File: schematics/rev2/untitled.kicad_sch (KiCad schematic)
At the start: 94 parts, among them SW1 KS-33, SW10 KS-33, SW11 KS-33, SW12 KS-33, SW13 KS-33, SW14 KS-33, SW15 KS-33, SW16 KS-33, SW17 KS-33, SW18 KS-33, SW19 KS-33, SW2 KS-33, SW20 KS-33, SW21 KS-33, SW22 KS-33, SW23 KS-33, SW24 KS-33, SW25 KS-33, SW26 KS-33, SW27 KS-33, SW28 KS-33, SW29 KS-33, SW3 KS-33, SW30 KS-33, SW31 KS-33, SW32 KS-33, SW33 KS-33, SW34 KS-33, SW35 KS-33, SW36 KS-33, SW37 KS-33, SW38 KS-33, SW39 KS-33, SW4 KS-33, SW40 KS-33, SW41 KS-33, SW42 KS-33, SW43 KS-33, SW44 KS-33, SW45 KS-33, SW46 KS-33, SW48 KS-33, SW5 KS-33, SW6 KS-33, SW7 KS-33, SW8 KS-33, SW9 KS-33

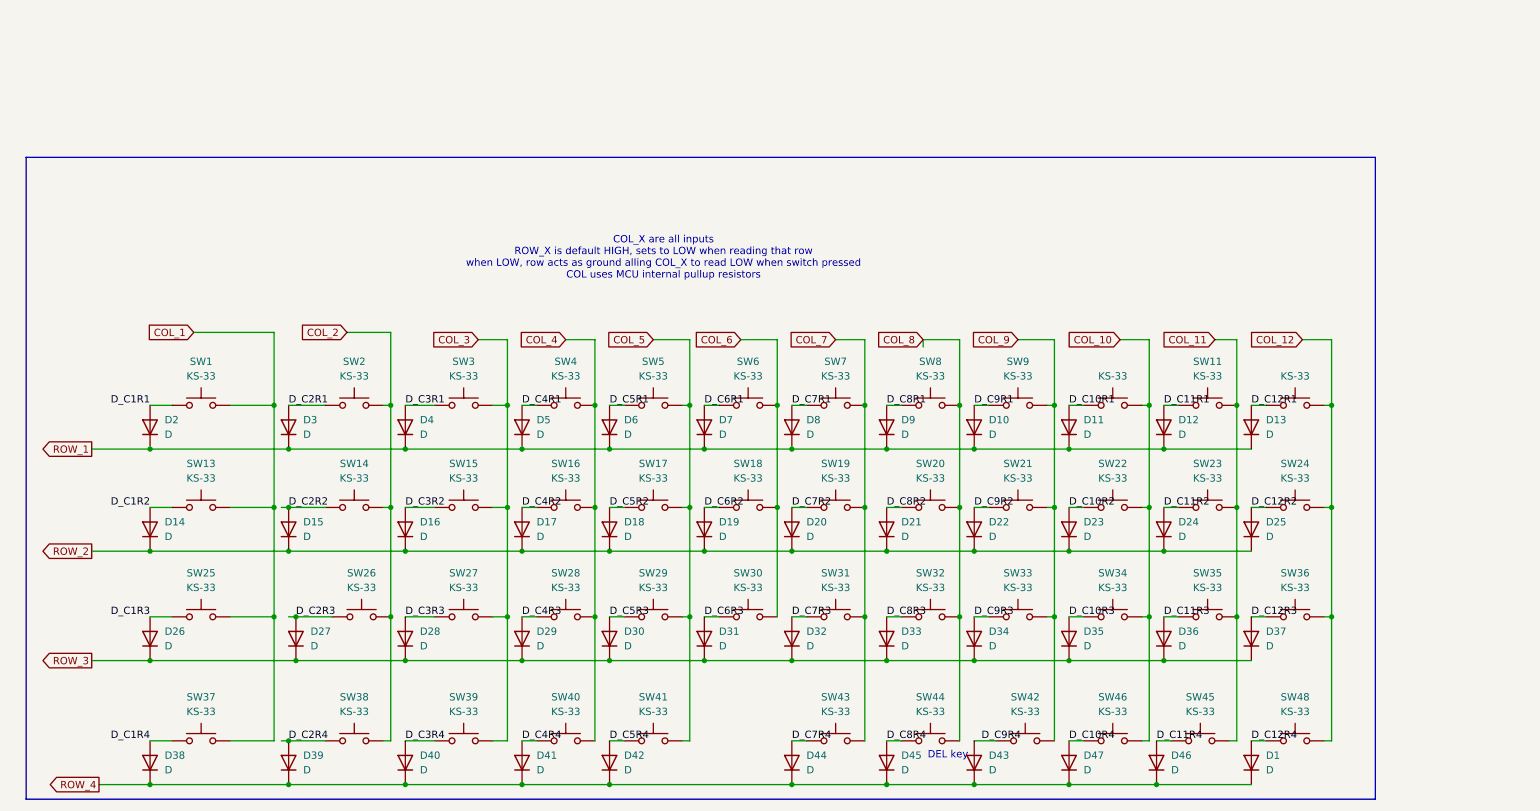
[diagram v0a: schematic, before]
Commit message: Update schematic and board layout
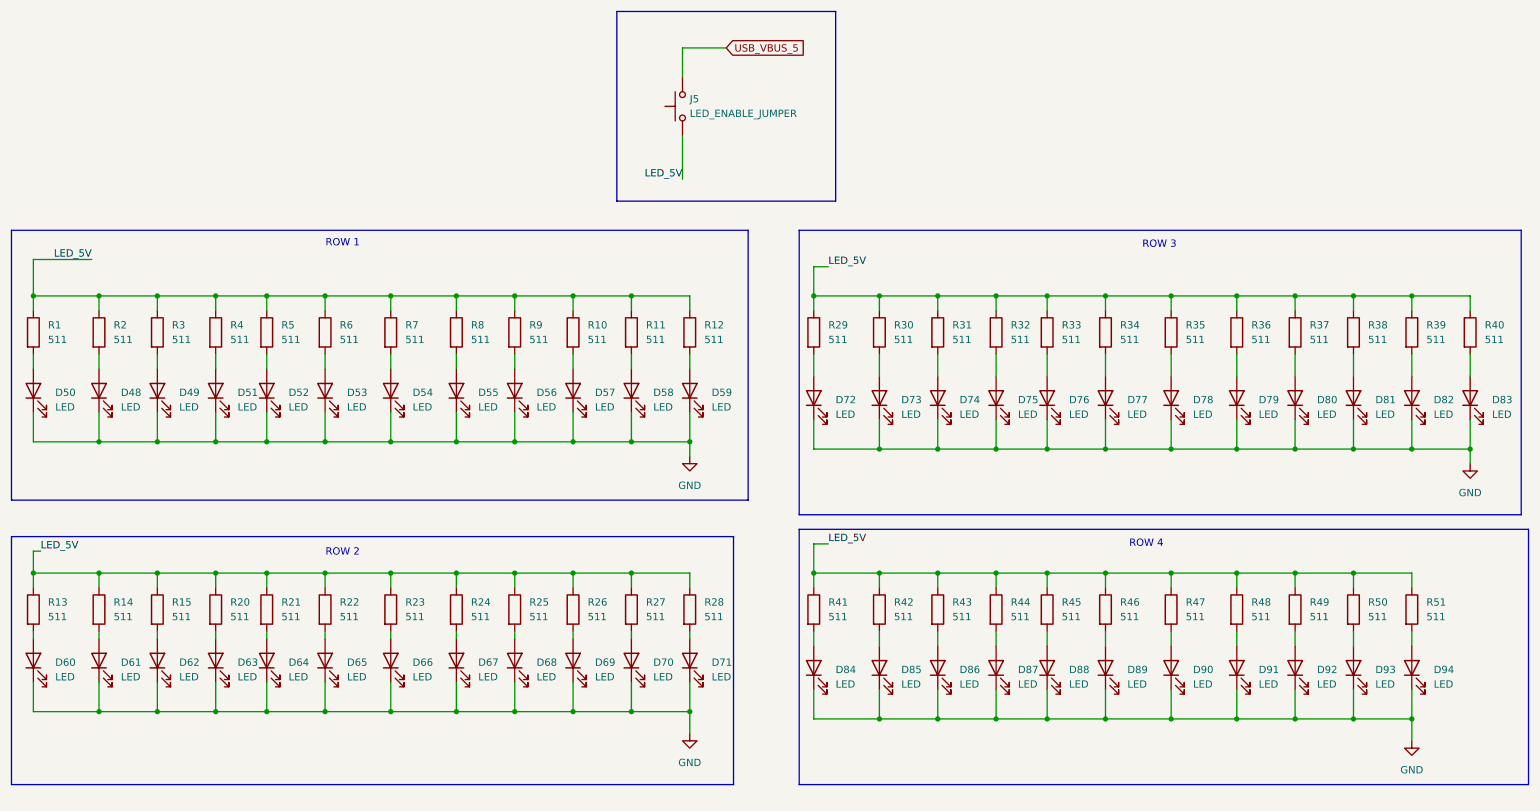
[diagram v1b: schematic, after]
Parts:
- removed D1, D10, D11, D12, D13, D14, D15, D16, D17, D18, D19, D2, D20, D21, D22, D23, D24, D25, D26, D27, D28, D29, D3, D30, D31, D32, D33, D34, D35, D36, D37, D38, D39, D4, D40, D41, D42, D43, D44, D45, D46, D47, D5, D6, D7, D8, D9: D, Diode_SMD:D_SOD-123, symbol Device:D
- removed SW1, SW10, SW11, SW12, SW13, SW14, SW15, SW16, SW17, SW18, SW19, SW2, SW20, SW21, SW22, SW23, SW24, SW25, SW26, SW27, SW28, SW29, SW3, SW30, SW31, SW32, SW33, SW34, SW35, SW36, SW37, SW38, SW39, SW4, SW40, SW41, SW42, SW43, SW44, SW45, SW46, SW48, SW5, SW6, SW7, SW8, SW9: KS-33, Library:Cherry MX switch, symbol Switches:Gateron_KS-33
- added D48, D49, D50, D51, D52, D53, D54, D55, D56, D57, D58, D59, D60, D61, D62, D63, D64, D65, D66, D67, D68, D69, D70, D71, D72, D73, D74, D75, D76, D77, D78, D79, D80, D81, D82, D83, D84, D85, D86, D87, D88, D89, D90, D91, D92, D93, D94: LED, LED_SMD:LED_1206_3216Metric_Pad1.42x1.75mm_HandSolder, symbol Device:LED
- added J5: LED_ENABLE_JUMPER, Jumper:SolderJumper-2_P1.3mm_Open_Pad1.0x1.5mm, symbol Switches:SW_Push
- added R1, R10, R11, R12, R13, R14, R15, R2, R20, R21, R22, R23, R24, R25, R26, R27, R28, R29, R3, R30, R31, R32, R33, R34, R35, R36, R37, R38, R39, R4, R40, R41, R42, R43, R44, R45, R46, R47, R48, R49, R5, R50, R51, R6, R7, R8, R9: 511, Resistor_SMD:R_1206_3216Metric_Pad1.30x1.75mm_HandSolder, symbol Device:R
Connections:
- new net: D78.2 (A), R35.2
- new net: D93.2 (A), R50.2
- new net: D82.2 (A), R39.2
- new net: D55.2 (A), R8.2
- new net: D53.2 (A), R6.2
- new net: D89.2 (A), R46.2
- new net: D69.2 (A), R26.2
- new net: D56.2 (A), R9.2
- new net: D68.2 (A), R25.2
- new net: D87.2 (A), R44.2
- new net: D70.2 (A), R27.2
- new net: D85.2 (A), R42.2
- new net: D75.2 (A), R32.2
- new net: D76.2 (A), R33.2
- new net: D72.2 (A), R29.2
- new net: D86.2 (A), R43.2
- new net: D71.2 (A), R28.2
- new net: D66.2 (A), R23.2
- new net: D51.2 (A), R4.2
- new net: D90.2 (A), R47.2
- new net: D81.2 (A), R38.2
- new net: D52.2 (A), R5.2
- new net: D83.2 (A), R40.2
- new net: D50.2 (A), R1.2
- new net: D92.2 (A), R49.2
- new net: D61.2 (A), R14.2
- new net: D49.2 (A), R3.2
- new net: D65.2 (A), R22.2
- new net: D88.2 (A), R45.2
- new net: D48.2 (A), R2.2
- new net: D77.2 (A), R34.2
- new net: D59.2 (A), R12.2
- new net: D80.2 (A), R37.2
- new net: D54.2 (A), R7.2
- new net: D94.2 (A), R51.2
- new net: D60.2 (A), R13.2
- new net: D84.2 (A), R41.2
- new net: D79.2 (A), R36.2
- new net: D64.2 (A), R21.2
- new net: D58.2 (A), R11.2
- new net: D91.2 (A), R48.2
- new net: D62.2 (A), R15.2
- new net: D57.2 (A), R10.2
- new net: D67.2 (A), R24.2
- new net: D73.2 (A), R30.2
- new net: D74.2 (A), R31.2
- new net: D63.2 (A), R20.2
- new net GND: D48.1 (K), D49.1 (K), D50.1 (K), D51.1 (K), D52.1 (K), D53.1 (K), D54.1 (K), D55.1 (K), D56.1 (K), D57.1 (K), D58.1 (K), D59.1 (K), D60.1 (K), D61.1 (K), D62.1 (K), D63.1 (K), D64.1 (K), D65.1 (K), D66.1 (K), D67.1 (K), D68.1 (K), D69.1 (K), D70.1 (K), D71.1 (K), D72.1 (K), D73.1 (K), D74.1 (K), D75.1 (K), D76.1 (K), D77.1 (K), D78.1 (K), D79.1 (K), D80.1 (K), D81.1 (K), D82.1 (K), D83.1 (K), D84.1 (K), D85.1 (K), D86.1 (K), D87.1 (K), D88.1 (K), D89.1 (K), D90.1 (K), D91.1 (K), D92.1 (K), D93.1 (K), D94.1 (K)
- new net LED_5V: J5.1, R1.1, R10.1, R11.1, R12.1, R13.1, R14.1, R15.1, R2.1, R20.1, R21.1, R22.1, R23.1, R24.1, R25.1, R26.1, R27.1, R28.1, R29.1, R3.1, R30.1, R31.1, R32.1, R33.1, R34.1, R35.1, R36.1, R37.1, R38.1, R39.1, R4.1, R40.1, R41.1, R42.1, R43.1, R44.1, R45.1, R46.1, R47.1, R48.1, R49.1, R5.1, R50.1, R51.1, R6.1, R7.1, R8.1, R9.1
- new net USB_VBUS_5: J5.2
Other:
- note added: "ROW 1"
- note added: "ROW 2"
- note added: "ROW 3"
- note added: "ROW 4"
- note removed: "COL_X are all inputs ROW_X is default HIGH, sets to LOW when reading that row when LOW, row acts as ground alling COL_X to read LOW when switch pressed COL uses MCU internal pullup resistors"
- note removed: "DEL key"
